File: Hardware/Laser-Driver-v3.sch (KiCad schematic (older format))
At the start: 16 parts, among them J1 Screw_Terminal_01x02, J2 74650074R, J5 74650074R, Q1 IRFP4568PbF, Q2 PSMN0R7-25YLD, U1 OPA2354AIDDA

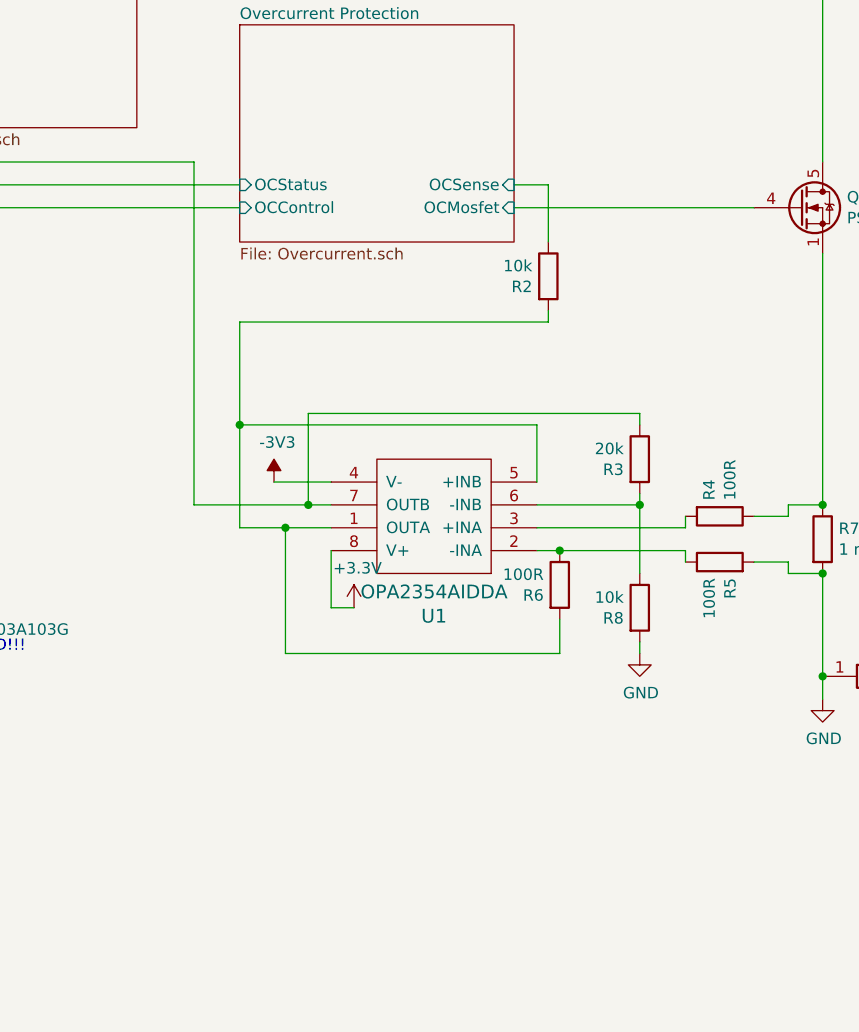
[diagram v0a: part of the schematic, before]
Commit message: swapped current sensing opamps for better routing
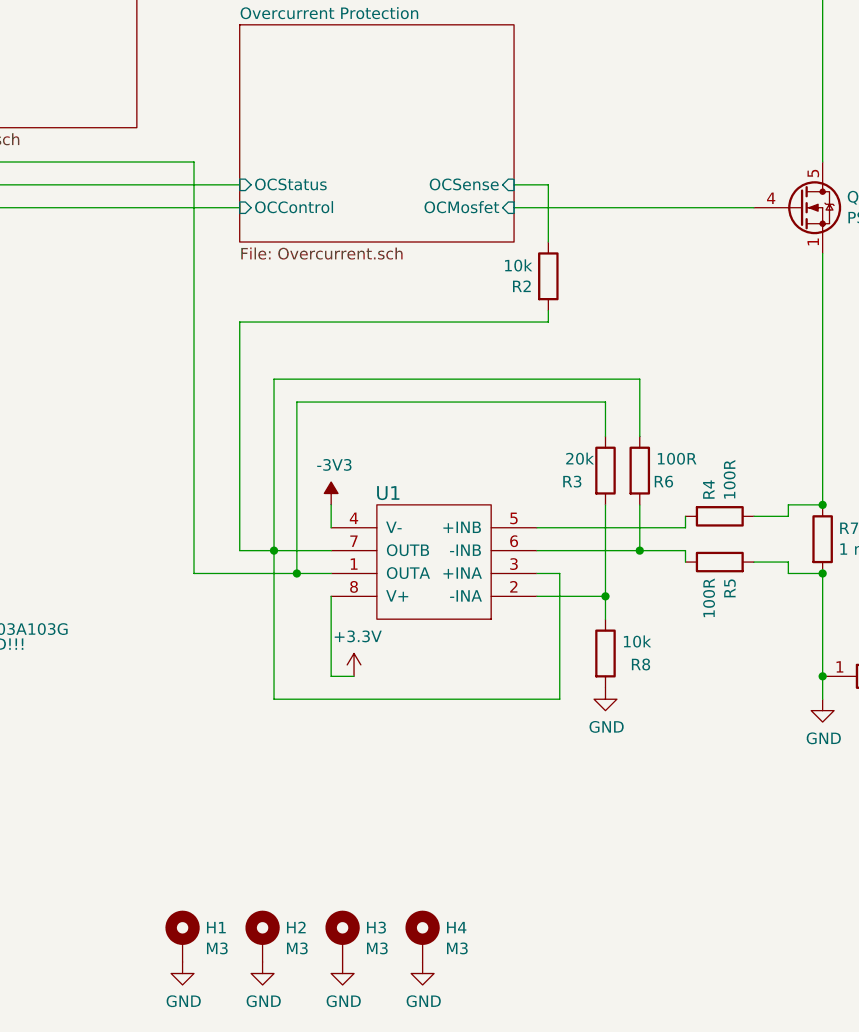
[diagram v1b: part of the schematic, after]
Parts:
- added H1, H2, H3, H4: M3, MountingHole:MountingHole_3.2mm_M3_Pad_Via, symbol Mechanical:MountingHole_Pad
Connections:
- net GND: now also H1.1, H2.1, H3.1, H4.1
- net Teensy/ADC-SHUNT: now also U1.1 (OUTA); no longer U1.7 (OUTB)
- net at R4.2: now also U1.5 (+INB); no longer U1.3 (+INA)
- net at R3.2, R8.1: now also U1.2 (-INA); no longer U1.6 (-INB)
- new net: R5.1, R6.2, U1.6 (-INB)
- new net: R2.2, R6.1, U1.3 (+INA), U1.7 (OUTB)
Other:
- moved on the sheet: R3, R6, R8, U1
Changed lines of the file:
@@
 	7500 3900 6450 3900
-$Comp
-L OS-LD:OPA2354 U1
-U 1 1 5F275BCA
-P 6350 5550
-F 0 "U1" H 6600 5687 60  0000 C CNN
-F 1 "OPA2354AIDDA" H 6600 5581 60  0000 C CNN
-F 2 "Package_SO:SOIC-8-1EP_3.9x4.9mm_P1.27mm_EP2.29x3mm" H 6400 5550 60  0001 C CNN
-F 3 "" H 6400 5550 60  0001 C CNN
-	1    6350 5550
-	-1   0    0    1
-$EndComp
 $Comp
 L Device:R R4
@@
 	7200 5300 7200 5250
 Wire Wire Line
-	6550 5400 6650 5400
-Wire Wire Line
 	7200 5400 7200 5450
-$Comp
-L Device:R R6
-U 1 1 5F25607D
-P 6650 5550
-F 0 "R6" H 6580 5504 50  0000 R CNN
-F 1 "100R" H 6580 5595 50  0000 R CNN
-F 2 "Resistor_SMD:R_0603_1608Metric" V 6580 5550 50  0001 C CNN
-F 3 "~" H 6650 5550 50  0001 C CNN
-	1    6650 5550
-	1    0    0    -1
-$EndComp
-Connection ~ 6650 5400
-Wire Wire Line
-	6650 5700 6650 5850
-Wire Wire Line
-	6650 5850 5450 5850
-Wire Wire Line
-	5450 5850 5450 5300
-Wire Wire Line
-	5450 5300 5650 5300
-$Comp
-L power:-3V3 #PWR0101
-U 1 1 5F7D57D9
-P 5400 5100
-F 0 "#PWR0101" H 5400 5200 50  0001 C CNN
-F 1 "-3V3" H 5415 5273 50  0000 C CNN
-F 2 "" H 5400 5100 50  0001 C CNN
-F 3 "" H 5400 5100 50  0001 C CNN
-	1    5400 5100
-	1    0    0    -1
-$EndComp
-Wire Wire Line
-	5400 5100 5650 5100
 $Comp
 L power:+3.3V #PWR0102
 U 1 1 5F7DD72F
-P 5750 5650
-F 0 "#PWR0102" H 5750 5500 50  0001 C CNN
-F 1 "+3.3V" H 5765 5823 50  0000 C CNN
-F 2 "" H 5750 5650 50  0001 C CNN
-F 3 "" H 5750 5650 50  0001 C CNN
-	1    5750 5650
-	1    0    0    -1
-$EndComp
-Wire Wire Line
-	5750 5650 5650 5650
-Wire Wire Line
-	5650 5650 5650 5400
-Wire Wire Line
-	5450 5300 5250 5300
-Wire Wire Line
-	5250 5300 5250 4850
-Wire Wire Line
-	5250 4850 6550 4850
-Wire Wire Line
-	6550 4850 6550 5100
-Connection ~ 5450 5300
+P 5750 5950
+F 0 "#PWR0102" H 5750 5800 50  0001 C CNN
+F 1 "+3.3V" H 5765 6123 50  0000 C CNN
+F 2 "" H 5750 5950 50  0001 C CNN
+F 3 "" H 5750 5950 50  0001 C CNN
+	1    5750 5950
+	1    0    0    -1
+$EndComp
 Wire Wire Line
 	6550 5300 7200 5300
-Wire Wire Line
-	6650 5400 7200 5400
 $Comp
 L Device:R R3
 U 1 1 5F800785
-P 7000 5000
-F 0 "R3" H 6930 4954 50  0000 R CNN
-F 1 "20k" H 6930 5045 50  0000 R CNN
-F 2 "Resistor_SMD:R_0603_1608Metric" V 6930 5000 50  0001 C CNN
-F 3 "~" H 7000 5000 50  0001 C CNN
-	1    7000 5000
+P 6850 5050
+F 0 "R3" H 6750 5000 50  0000 R CNN
+F 1 "20k" H 6800 5100 50  0000 R CNN
+F 2 "Resistor_SMD:R_0603_1608Metric" V 6780 5050 50  0001 C CNN
+F 3 "~" H 6850 5050 50  0001 C CNN
+	1    6850 5050
 	1    0    0    -1
 $EndComp
@@
 L Device:R R8
 U 1 1 5F8011C2
-P 7000 5650
-F 0 "R8" H 6930 5604 50  0000 R CNN
-F 1 "10k" H 6930 5695 50  0000 R CNN
-F 2 "Resistor_SMD:R_0603_1608Metric" V 6930 5650 50  0001 C CNN
-F 3 "~" H 7000 5650 50  0001 C CNN
-	1    7000 5650
+P 6850 5850
+F 0 "R8" H 7050 5800 50  0000 R CNN
+F 1 "10k" H 7050 5900 50  0000 R CNN
+F 2 "Resistor_SMD:R_0603_1608Metric" V 6780 5850 50  0001 C CNN
+F 3 "~" H 6850 5850 50  0001 C CNN
+	1    6850 5850
 	1    0    0    -1
 $EndComp
@@
 L power:GND #PWR0103
 U 1 1 5F801827
-P 7000 5850
-F 0 "#PWR0103" H 7000 5600 50  0001 C CNN
-F 1 "GND" H 7005 5677 50  0000 C CNN
-F 2 "" H 7000 5850 50  0001 C CNN
-F 3 "" H 7000 5850 50  0001 C CNN
-	1    7000 5850
-	1    0    0    -1
-$EndComp
-Wire Wire Line
-	7000 5500 7000 5200
-Wire Wire Line
-	6550 5200 7000 5200
-Connection ~ 7000 5200
-Wire Wire Line
-	7000 5200 7000 5150
-Wire Wire Line
-	5650 5200 5550 5200
-Wire Wire Line
-	5550 5200 5550 4800
-Wire Wire Line
-	5550 4800 7000 4800
-Wire Wire Line
-	7000 4800 7000 4850
-Wire Wire Line
-	5050 5200 5550 5200
-Wire Wire Line
-	5050 3700 5050 5200
-Connection ~ 5550 5200
-Wire Wire Line
-	7000 5800 7000 5850
+P 6850 6000
+F 0 "#PWR0103" H 6850 5750 50  0001 C CNN
+F 1 "GND" H 6855 5827 50  0000 C CNN
+F 2 "" H 6850 6000 50  0001 C CNN
+F 3 "" H 6850 6000 50  0001 C CNN
+	1    6850 6000
+	1    0    0    -1
+$EndComp
 $Comp
 L Device:R R2
@@
 	6600 4400 5250 4400
 Wire Wire Line
-	5250 4400 5250 4850
-Connection ~ 5250 4850
-Wire Wire Line
 	2900 4550 2900 4900
 $Comp
@@
 	7650 5200 7650 5250
 Connection ~ 7800 5200
+$Comp
+L Mechanical:MountingHole_Pad H1
+U 1 1 6014D0CD
+P 5000 7100
+F 0 "H1" H 5100 7149 50  0000 L CNN
+F 1 "M3" H 5100 7058 50  0000 L CNN
+F 2 "MountingHole:MountingHole_3.2mm_M3_Pad_Via" H 5000 7100 50  0001 C CNN
+F 3 "~" H 5000 7100 50  0001 C CNN
+	1    5000 7100
+	1    0    0    -1
+$EndComp
+$Comp
+L Mechanical:MountingHole_Pad H2
+U 1 1 6014DDE2
+P 5350 7100
+F 0 "H2" H 5450 7149 50  0000 L CNN
+F 1 "M3" H 5450 7058 50  0000 L CNN
+F 2 "MountingHole:MountingHole_3.2mm_M3_Pad_Via" H 5350 7100 50  0001 C CNN
+F 3 "~" H 5350 7100 50  0001 C CNN
+	1    5350 7100
+	1    0    0    -1
+$EndComp
+$Comp
+L Mechanical:MountingHole_Pad H3
+U 1 1 6014DF82
+P 5700 7100
+F 0 "H3" H 5800 7149 50  0000 L CNN
+F 1 "M3" H 5800 7058 50  0000 L CNN
+F 2 "MountingHole:MountingHole_3.2mm_M3_Pad_Via" H 5700 7100 50  0001 C CNN
+F 3 "~" H 5700 7100 50  0001 C CNN
+	1    5700 7100
+	1    0    0    -1
+$EndComp
+$Comp
+L Mechanical:MountingHole_Pad H4
+U 1 1 6014E1EB
+P 6050 7100
+F 0 "H4" H 6150 7149 50  0000 L CNN
+F 1 "M3" H 6150 7058 50  0000 L CNN
+F 2 "MountingHole:MountingHole_3.2mm_M3_Pad_Via" H 6050 7100 50  0001 C CNN
+F 3 "~" H 6050 7100 50  0001 C CNN
+	1    6050 7100
+	1    0    0    -1
+$EndComp
+$Comp
+L power:GND #PWR052
+U 1 1 6014EB9A
+P 6050 7200
+F 0 "#PWR052" H 6050 6950 50  0001 C CNN
+F 1 "GND" H 6055 7027 50  0000 C CNN
+F 2 "" H 6050 7200 50  0001 C CNN
+F 3 "" H 6050 7200 50  0001 C CNN
+	1    6050 7200
+	1    0    0    -1
+$EndComp
+$Comp
+L power:GND #PWR051
+U 1 1 6014F236
+P 5700 7200
+F 0 "#PWR051" H 5700 6950 50  0001 C CNN
+F 1 "GND" H 5705 7027 50  0000 C CNN
+F 2 "" H 5700 7200 50  0001 C CNN
+F 3 "" H 5700 7200 50  0001 C CNN
+	1    5700 7200
+	1    0    0    -1
+$EndComp
+$Comp
+L power:GND #PWR050
+U 1 1 6014F447
+P 5350 7200
+F 0 "#PWR050" H 5350 6950 50  0001 C CNN
+F 1 "GND" H 5355 7027 50  0000 C CNN
+F 2 "" H 5350 7200 50  0001 C CNN
+F 3 "" H 5350 7200 50  0001 C CNN
+	1    5350 7200
+	1    0    0    -1
+$EndComp
+$Comp
+L power:GND #PWR049
+U 1 1 6014F621
+P 5000 7200
+F 0 "#PWR049" H 5000 6950 50  0001 C CNN
+F 1 "GND" H 5005 7027 50  0000 C CNN
+F 2 "" H 5000 7200 50  0001 C CNN
+F 3 "" H 5000 7200 50  0001 C CNN
+	1    5000 7200
+	1    0    0    -1
+$EndComp
+$Comp
+L power:-3V3 #PWR0101
+U 1 1 5F7D57D9
+P 5650 5200
+F 0 "#PWR0101" H 5650 5300 50  0001 C CNN
+F 1 "-3V3" H 5665 5373 50  0000 C CNN
+F 2 "" H 5650 5200 50  0001 C CNN
+F 3 "" H 5650 5200 50  0001 C CNN
+	1    5650 5200
+	1    0    0    -1
+$EndComp
+$Comp
+L OS-LD:OPA2354 U1
+U 1 1 5F275BCA
+P 6350 5750
+F 0 "U1" H 6800 5150 60  0000 C CNN
+F 1 "OPA2354AIDDA" H 6600 5781 60  0001 C CNN
+F 2 "Package_SO:SOIC-8-1EP_3.9x4.9mm_P1.27mm_EP2.29x3mm" H 6400 5750 60  0001 C CNN
+F 3 "" H 6400 5750 60  0001 C CNN
+	1    6350 5750
+	-1   0    0    1
+$EndComp
+Wire Wire Line
+	5250 5400 5400 5400
+Wire Wire Line
+	6650 5500 6550 5500
+$Comp
+L Device:R R6
+U 1 1 5F25607D
+P 7000 5050
+F 0 "R6" H 7150 5000 50  0000 R CNN
+F 1 "100R" H 7250 5100 50  0000 R CNN
+F 2 "Resistor_SMD:R_0603_1608Metric" V 6930 5050 50  0001 C CNN
+F 3 "~" H 7000 5050 50  0001 C CNN
+	1    7000 5050
+	1    0    0    -1
+$EndComp
+Wire Wire Line
+	6850 5200 6850 5600
+Wire Wire Line
+	6550 5600 6850 5600
+Connection ~ 6850 5600
+Wire Wire Line
+	6850 5600 6850 5700
+Wire Wire Line
+	5650 5500 5500 5500
+Wire Wire Line
+	5500 5500 5500 4750
+Wire Wire Line
+	5500 4750 6850 4750
+Wire Wire Line
+	6850 4750 6850 4900
+Wire Wire Line
+	5650 5200 5650 5300
+Wire Wire Line
+	5650 5950 5650 5600
+Wire Wire Line
+	6550 5400 7000 5400
+Wire Wire Line
+	7000 5200 7000 5400
+Connection ~ 7000 5400
+Wire Wire Line
+	7000 5400 7200 5400
+Wire Wire Line
+	7000 4900 7000 4650
+Wire Wire Line
+	5400 4650 5400 5400
+Connection ~ 5400 5400
+Wire Wire Line
+	5400 5400 5650 5400
+Wire Wire Line
+	5250 4400 5250 5400
+Wire Wire Line
+	5400 4650 7000 4650
+Wire Wire Line
+	6650 5500 6650 6050
+Wire Wire Line
+	6650 6050 5400 6050
+Wire Wire Line
+	5400 6050 5400 5400
+Wire Wire Line
+	5500 5500 5050 5500
+Wire Wire Line
+	5050 3700 5050 5500
+Connection ~ 5500 5500
+Wire Wire Line
+	5750 5950 5650 5950
 $EndSCHEMATC
